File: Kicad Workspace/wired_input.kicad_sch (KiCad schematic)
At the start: 38 parts, among them J1 NMJ4HFD2, J2 NMJ4HFD2, J3 NMJ6HFD2, J4 NMJ4HFD2, U2 PCM1863DBT, Y1 Crystal

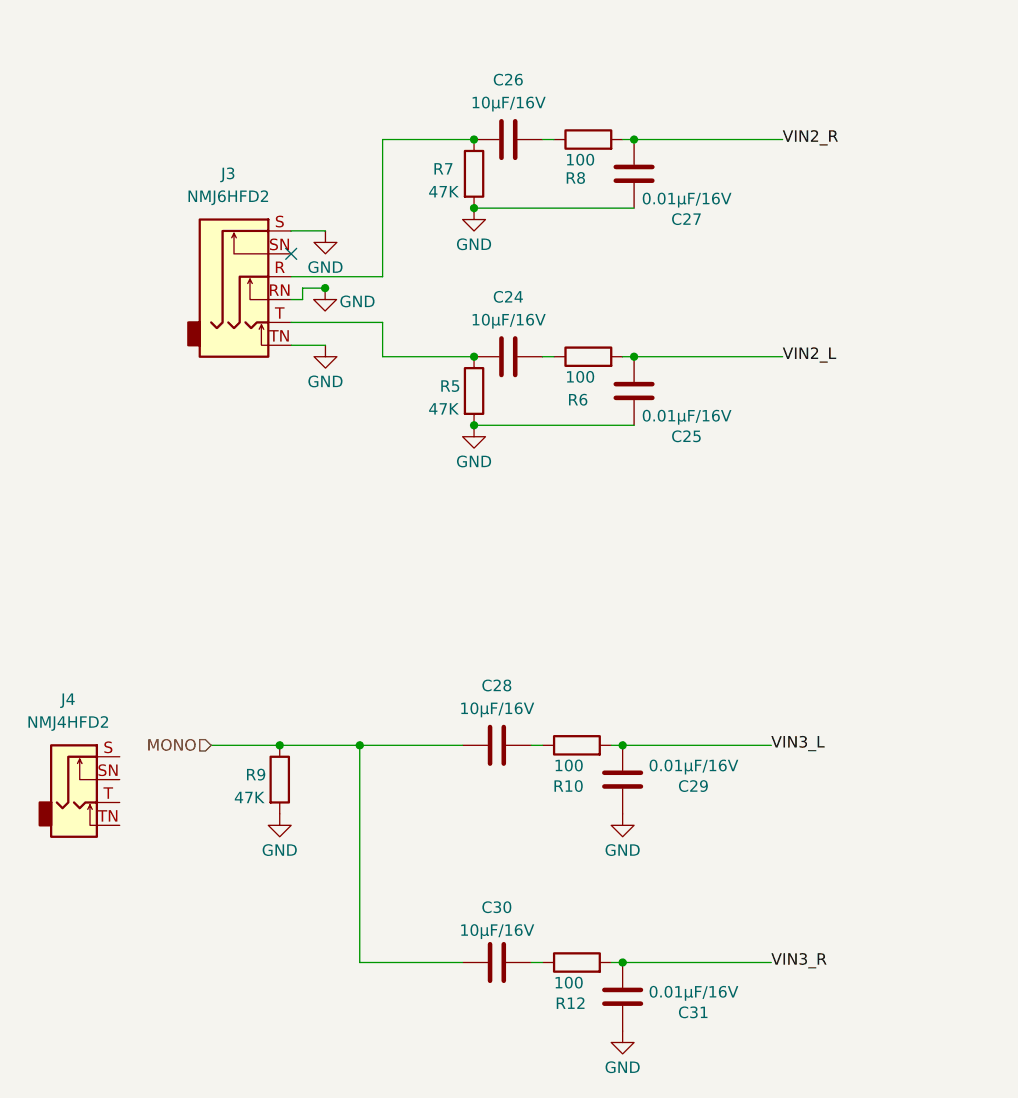
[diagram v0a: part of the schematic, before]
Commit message: feat: jack schematics
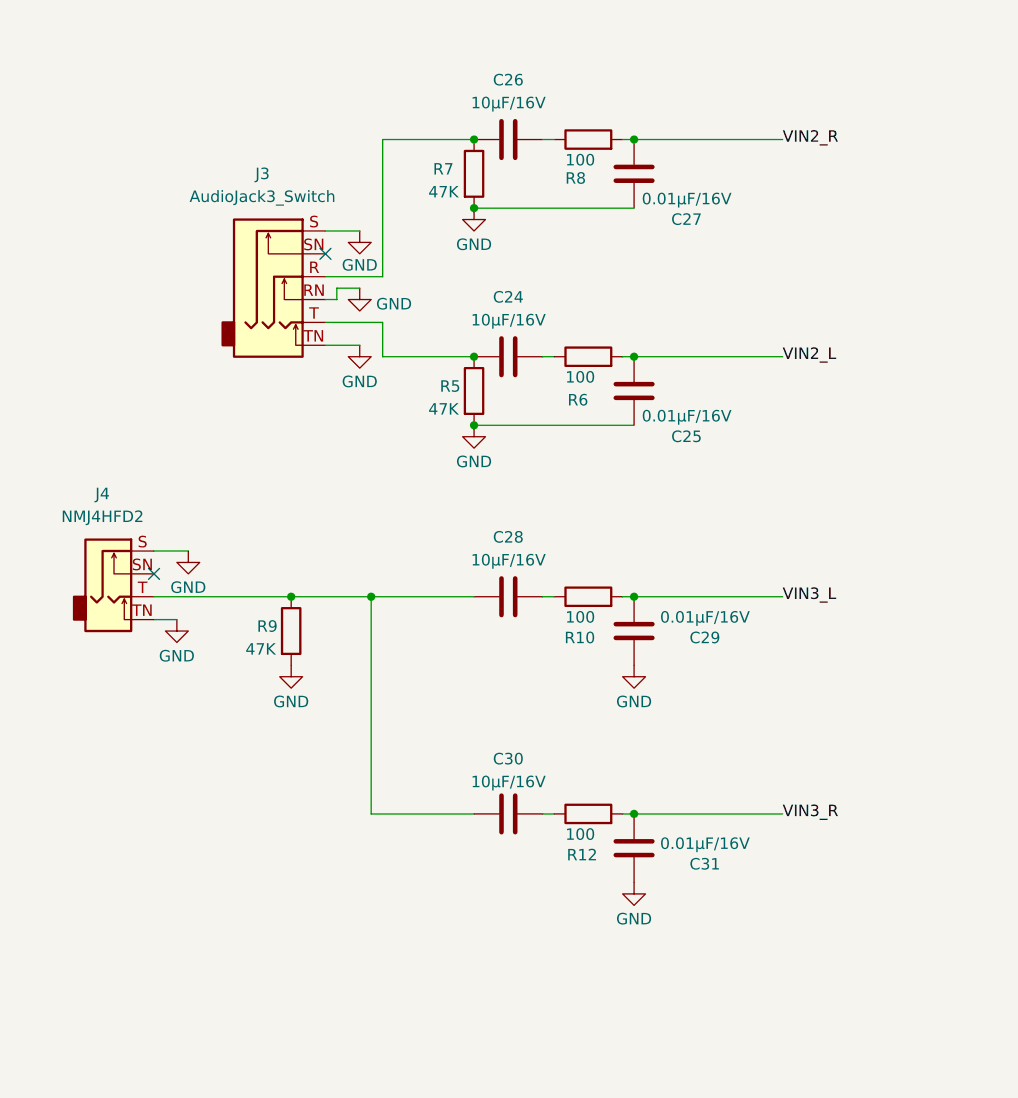
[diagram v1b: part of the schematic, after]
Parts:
- removed J3: NMJ6HFD2, Connector_Audio:Jack_6.35mm_Neutrik_NMJ6HFD2_Horizontal, symbol Connector_Audio:NMJ6HFD2
- added J3: AudioJack3_Switch, Connector_Audio:Jack_3.5mm_CUI_SJ1-3535NG_Horizontal, symbol Connector_Audio:AudioJack3_Switch
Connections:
- net MONO is gone; now on an unnamed net: C28.1, C30.1, R9.1
- net GND: now also J4.S, J4.TN, J3.RN, J3.S, J3.TN
- net at C26.1, R7.1: now also J3.R
- net at C24.1, R5.1: now also J3.T
- no-connect marks 10 -> 11
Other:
- moved on the sheet: C28, C29, C30, C31, J4, R10, R12, R9
